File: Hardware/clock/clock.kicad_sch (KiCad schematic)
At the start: 34 parts, among them J1 Barrel_Jack_Switch, J3 Conn_02x03_Odd_Even, Q1 BC817, Q2 BC817, SW1 PTH_RA_h7.5mm, U1 SBC18-11EGWA, U2 SBC18-11EGWA, U3 SBC18-11EGWA, U4 ESP32-WROOM-32, U5 SBC18-11EGWA, U6 MAX7221xNG, U7 AMS1117-3.3, U8 LM2596S-5

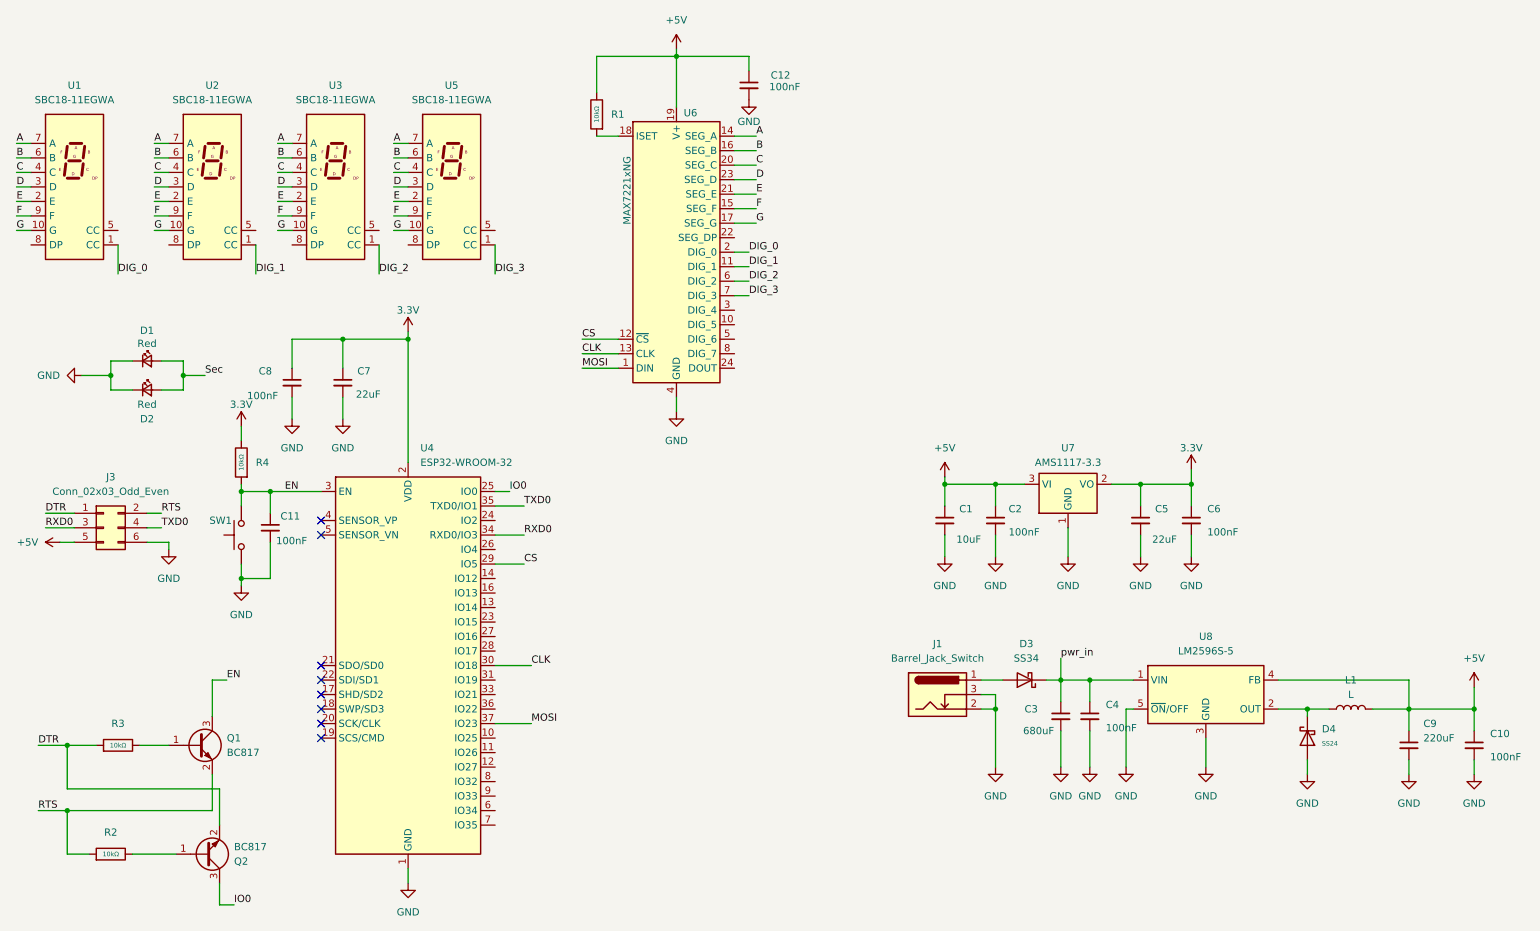
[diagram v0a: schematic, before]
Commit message: Updated README.md
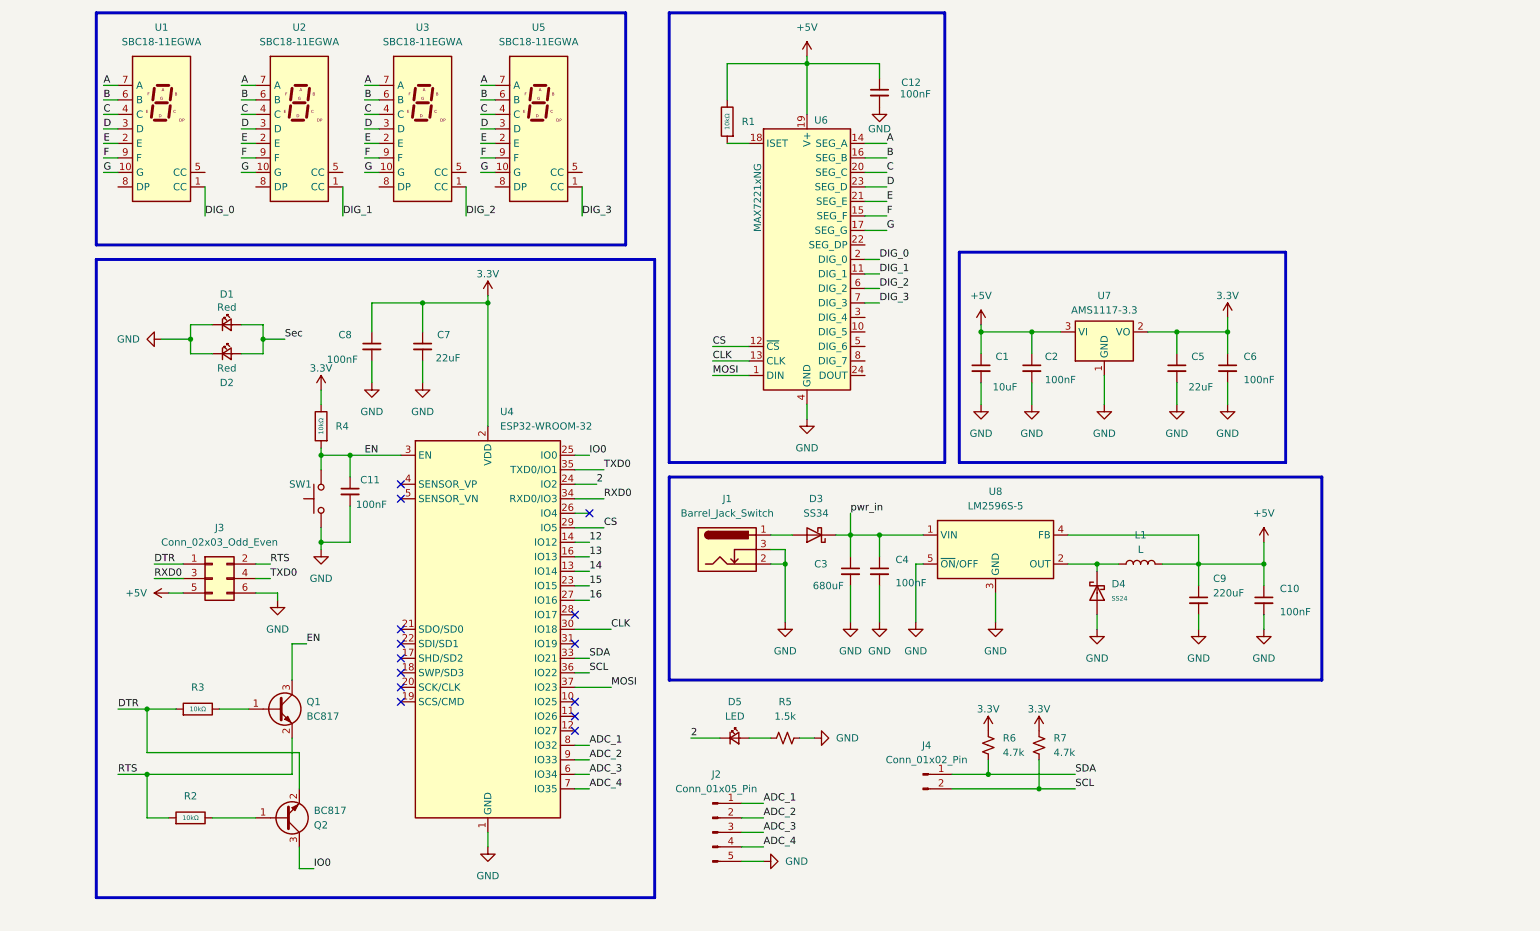
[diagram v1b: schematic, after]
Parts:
- added D5: LED, SparkFun-LED:LED_0603_1608Metric, symbol SparkFun-LED:LED
- added J2: Conn_01x05_Pin, Connector_PinHeader_2.54mm:PinHeader_1x05_P2.54mm_Vertical, symbol Connector:Conn_01x05_Pin
- added J4: Conn_01x02_Pin, Connector_PinHeader_2.00mm:PinHeader_1x02_P2.00mm_Vertical, symbol Connector:Conn_01x02_Pin
- added R5: 1.5k, SparkFun-Resistor:R_0603_1608Metric, symbol SparkFun-Resistor:1.5k_0603
- added R6, R7: 4.7k, SparkFun-Resistor:R_0603_1608Metric, symbol SparkFun-Resistor:4.7k_0603
- J3: footprint Connector_IDC:IDC-Header_2x03_P2.54mm_Horizontal -> Connector_PinHeader_2.54mm:PinHeader_1x06_P2.54mm_Vertical
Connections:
- net 3.3V: now also R6.2, R7.2
- net GND: now also J2.5 (Pin_5), R5.2
- net 14: now reaches U4.13 (IO14)
- net 12: now reaches U4.14 (IO12)
- net 13: now reaches U4.16 (IO13)
- net 15: now reaches U4.23 (IO15)
- net 2: now reaches U4.24 (IO2)
- net 2: now also D5.1 (K)
- net 16: now reaches U4.27 (IO16)
- net SDA: now reaches U4.33 (IO21)
- net SDA: now also J4.1 (Pin_1), R6.1
- net SCL: now reaches U4.36 (IO22)
- net SCL: now also J4.2 (Pin_2), R7.1
- net ADC_3: now reaches U4.6 (IO34)
- net ADC_3: now also J2.3 (Pin_3)
- net ADC_4: now reaches U4.7 (IO35)
- net ADC_4: now also J2.4 (Pin_4)
- net ADC_1: now reaches U4.8 (IO32)
- net ADC_1: now also J2.1 (Pin_1)
- net ADC_2: now reaches U4.9 (IO33)
- net ADC_2: now also J2.2 (Pin_2)
- new net: D5.2 (A), R5.1
- no-connect marks 8 -> 14
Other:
- moved on the sheet: C1, C10, C11, C12, C2, C3, C4, C5, C6, C7, C8, C9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
